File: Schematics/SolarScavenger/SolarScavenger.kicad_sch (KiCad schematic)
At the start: 52 parts, among them J1 SolarConnector, J10 CH1_IN, J11 CH2_IN, J12 CH3_IN, J13 CH4_IN, J14 CH1_OUT, J15 CH2_OUT, J16 CH3_OUT, J17 CH4_OUT, J2 PROGRAMMING, J3 BatteryPack, J4 ESC_PWM_CONTROL, J5 ESC_connector, J6 Micro_SD_Card, J7 RUDDER_POT, J8 THROTTLE_POt, Q1 IRLML2502, Q2 IRLML2502, U1 DS18B20, U2 4N25, U3 AP1117-33, U4 ESP32-WROOM-E, U5 INA219AxD

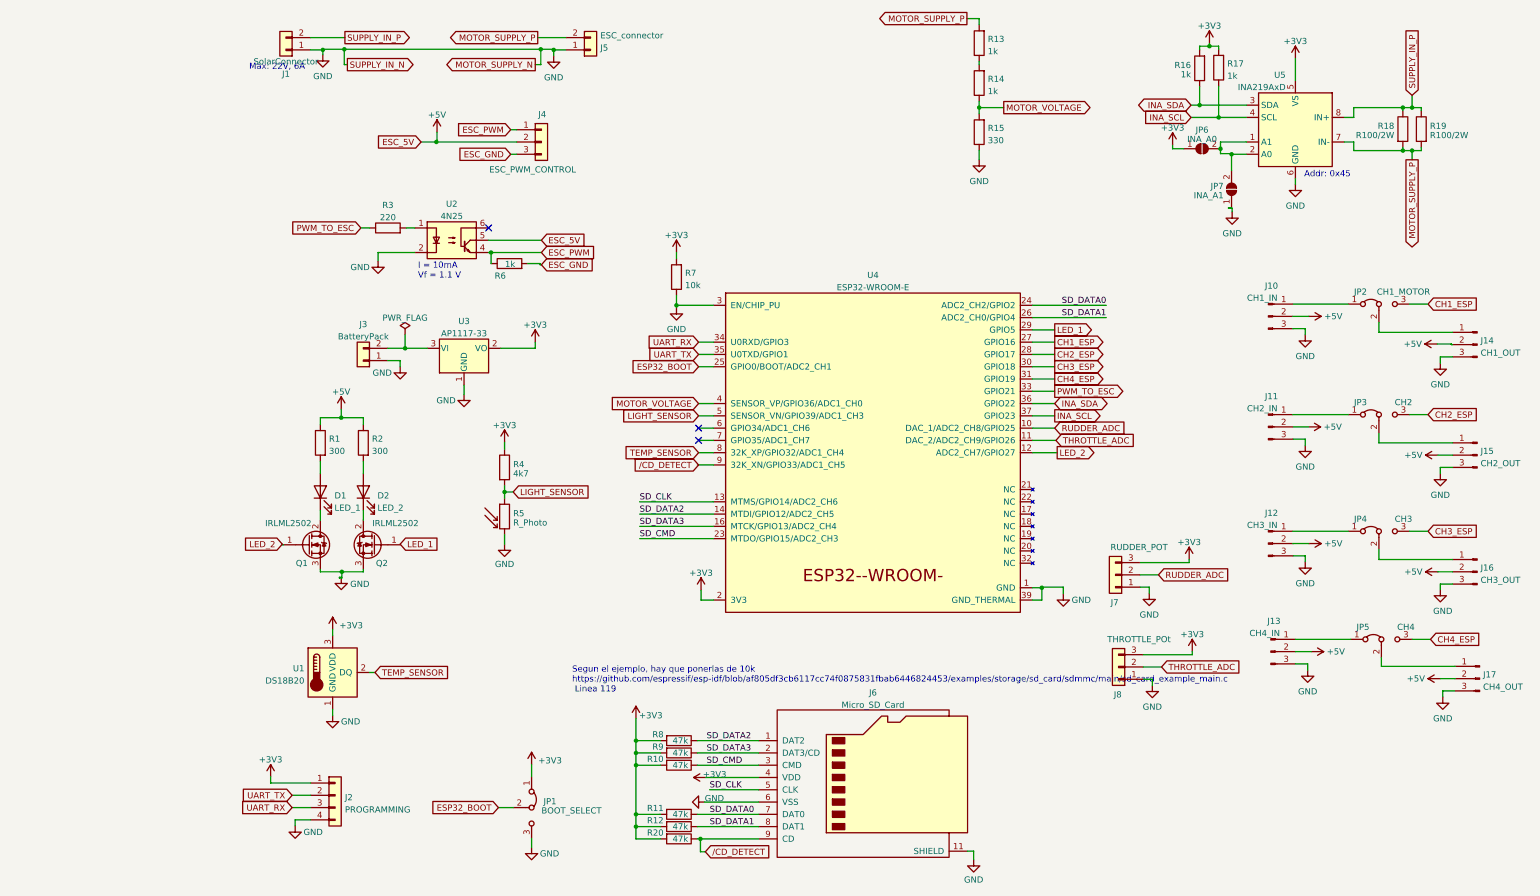
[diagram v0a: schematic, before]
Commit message: PCB v1.1
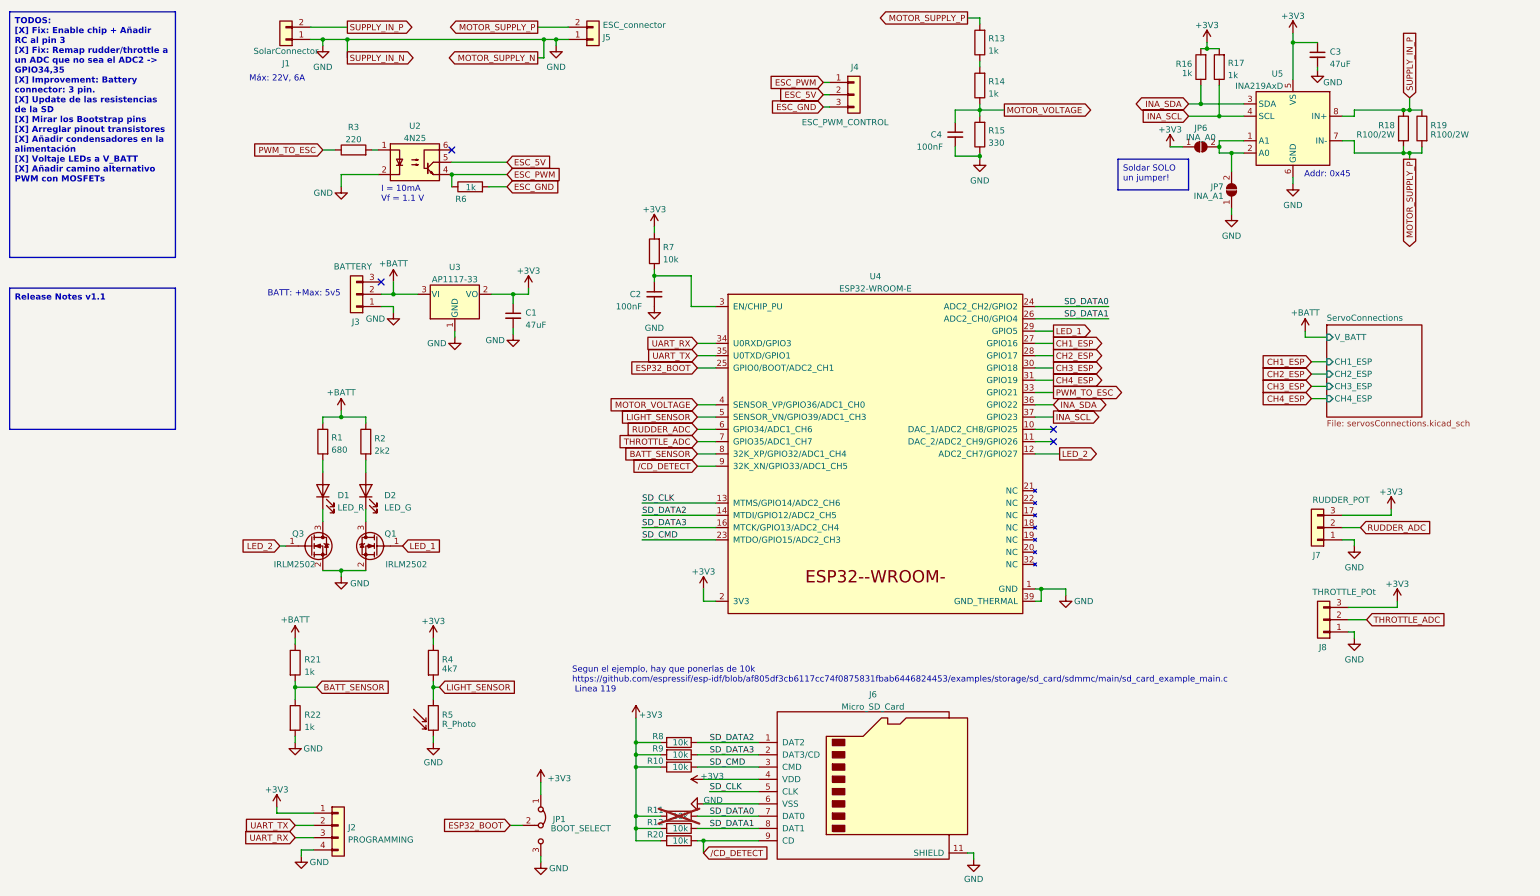
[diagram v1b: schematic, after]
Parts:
- removed J10: CH1_IN, Connector_PinHeader_2.54mm:PinHeader_1x03_P2.54mm_Vertical, symbol Connector:Conn_01x03_Male
- removed J11: CH2_IN, Connector_PinHeader_2.54mm:PinHeader_1x03_P2.54mm_Vertical, symbol Connector:Conn_01x03_Male
- removed J12: CH3_IN, Connector_PinHeader_2.54mm:PinHeader_1x03_P2.54mm_Vertical, symbol Connector:Conn_01x03_Male
- removed J13: CH4_IN, Connector_PinHeader_2.54mm:PinHeader_1x03_P2.54mm_Vertical, symbol Connector:Conn_01x03_Male
- removed J14: CH1_OUT, Connector_PinHeader_2.54mm:PinHeader_1x03_P2.54mm_Vertical, symbol Connector:Conn_01x03_Male
- removed J15: CH2_OUT, Connector_PinHeader_2.54mm:PinHeader_1x03_P2.54mm_Vertical, symbol Connector:Conn_01x03_Male
- removed J16: CH3_OUT, Connector_PinHeader_2.54mm:PinHeader_1x03_P2.54mm_Vertical, symbol Connector:Conn_01x03_Male
- removed J17: CH4_OUT, Connector_PinHeader_2.54mm:PinHeader_1x03_P2.54mm_Vertical, symbol Connector:Conn_01x03_Male
- removed J3: BatteryPack, Connector_PinHeader_2.54mm:PinHeader_1x02_P2.54mm_Vertical, symbol Connector_Generic:Conn_01x02
- removed JP2: CH1_MOTOR, Connector_PinHeader_2.54mm:PinHeader_1x03_P2.54mm_Vertical, symbol Jumper:Jumper_3_Bridged12
- removed JP3: CH2, Connector_PinHeader_2.54mm:PinHeader_1x03_P2.54mm_Vertical, symbol Jumper:Jumper_3_Bridged12
- removed JP4: CH3, Connector_PinHeader_2.54mm:PinHeader_1x03_P2.54mm_Vertical, symbol Jumper:Jumper_3_Bridged12
- removed JP5: CH4, Connector_PinHeader_2.54mm:PinHeader_1x03_P2.54mm_Vertical, symbol Jumper:Jumper_3_Bridged12
- removed Q1, Q2: IRLML2502, Package_TO_SOT_SMD:SOT-23_Handsoldering, symbol Transistor_FET:IRLZ44N
- removed U1: DS18B20, Package_TO_SOT_THT:TO-92_Inline, symbol Sensor_Temperature:DS18B20
- added C1, C3: 47uF, Capacitor_SMD:C_1206_3216Metric_Pad1.33x1.80mm_HandSolder, symbol Device:C_Small
- added C2, C4: 100nF, Capacitor_SMD:C_1206_3216Metric_Pad1.33x1.80mm_HandSolder, symbol Device:C_Small
- added J3: BATTERY, Connector_PinHeader_2.54mm:PinHeader_1x03_P2.54mm_Vertical, symbol Connector_Generic:Conn_01x03
- added Q1, Q3: IRLM2502, Package_TO_SOT_SMD:SOT-23, symbol GluonLib:IRLM2502
- added R21, R22: 1k, Resistor_SMD:R_1206_3216Metric_Pad1.30x1.75mm_HandSolder, symbol Device:R
- D1: value LED_1 -> LED_R
- D2: value LED_2 -> LED_G
- R1: value 300 -> 680
- R10, R12, R20, R8, R9: value 47k -> 10k
- R11: value 47k -> 10k; now not fitted
- R2: value 300 -> 2k2
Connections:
- net +3V3: now also C1.1, C3.1
- net GND: now also C1.2, C2.2, C3.2, C4.2, J3.1 (Pin_1), Q1.2 (S), Q3.2 (S), R22.2; no longer R7.1, U4.3 (EN/CHIP_PU)
- net LED_1: now also Q1.1 (G)
- net LED_2: now also Q3.1 (G)
- net MOTOR_VOLTAGE: now also C4.1
- net RUDDER_ADC: now also U4.6 (GPIO34/ADC1_CH6); no longer U4.10 (DAC_1/ADC2_CH8/GPIO25)
- net THROTTLE_ADC: now also U4.7 (GPIO35/ADC1_CH7); no longer U4.11 (DAC_2/ADC2_CH9/GPIO26)
- net at D1.1 (K): now also Q3.3 (D)
- net +BATT: now reaches U3.3 (VI)
- net +BATT: now also R1.1, R2.1, J3.2 (Pin_2), R21.1
- net at D2.1 (K): now also Q1.3 (D)
- net +5V renamed ESC_5V
- net ESC_5V: no longer R1.1, R2.1
- net TEMP_SENSOR renamed BATT_SENSOR
- net BATT_SENSOR: now also R21.2, R22.1
- new net: C2.1, R7.1, U4.3 (EN/CHIP_PU)
- no-connect marks 3 -> 4
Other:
- added sheet ServoConnections (servosConnections.kicad_sch)
- note added: "BATT: +Max: 5v5"
- moved on the sheet: D1, D2, J1, J2, J4, J5, J7, J8, JP1, R1, R14, R15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
